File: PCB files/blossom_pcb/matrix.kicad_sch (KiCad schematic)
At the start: 136 parts, among them SW1 SW_Push, SW10 SW_Push, SW11 SW_Push, SW12 SW_Push, SW13 SW_Push, SW14 SW_Push, SW15 SW_Push, SW16 SW_Push, SW17 SW_Push, SW18 SW_Push, SW19 SW_Push, SW2 SW_Push, SW20 SW_Push, SW21 SW_Push, SW22 SW_Push, SW23 SW_Push, SW24 SW_Push, SW25 SW_Push, SW26 SW_Push, SW27 SW_Push, SW28 SW_Push, SW29 SW_Push, SW3 SW_Push, SW30 SW_Push, SW31 SW_Push, SW32 SW_Push, SW33 SW_Push, SW34 SW_Push, SW35 SW_Push, SW36 SW_Push, SW37 SW_Push, SW38 SW_Push, SW39 SW_Push, SW4 SW_Push, SW40 SW_Push, SW41 SW_Push, SW42 SW_Push, SW43 SW_Push, SW44 SW_Push, SW45 SW_Push, SW46 SW_Push, SW47 SW_Push, SW48 SW_Push, SW49 SW_Push, SW5 SW_Push, SW50 SW_Push, SW51 SW_Push, SW52 SW_Push, SW53 SW_Push, SW54 SW_Push, SW55 SW_Push, SW56 SW_Push, SW57 SW_Push, SW58 SW_Push, SW59 SW_Push, SW6 SW_Push, SW60 SW_Push, SW61 SW_Push, SW62 SW_Push, SW63 SW_Push, SW64 SW_Push, SW65 SW_Push, SW66 SW_Push, SW67 SW_Push, SW68 SW_Push, SW7 SW_Push, SW8 SW_Push, SW9 SW_Push

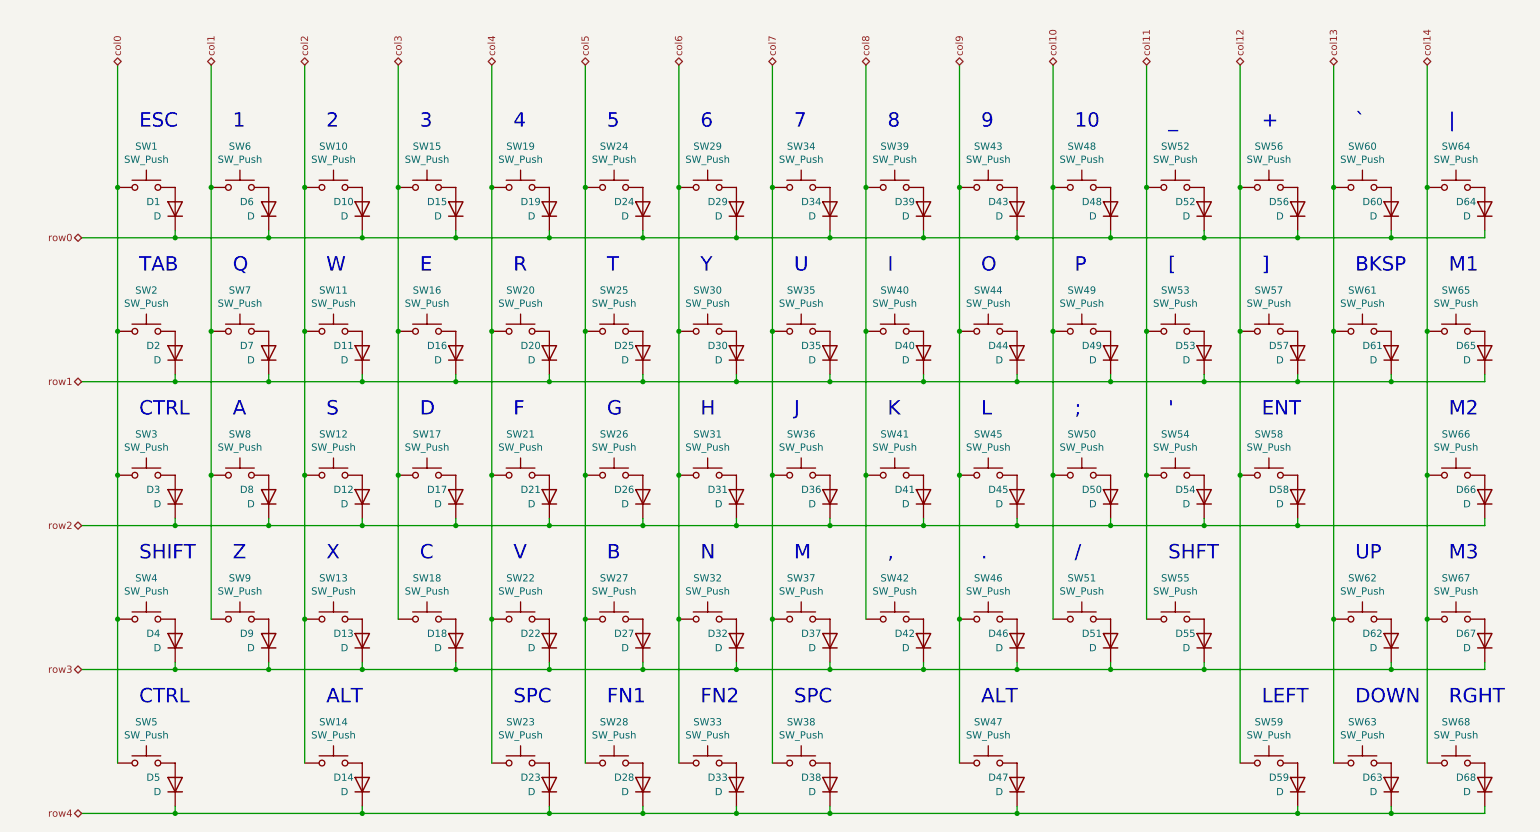
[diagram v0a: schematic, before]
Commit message: Almost doing stuffs
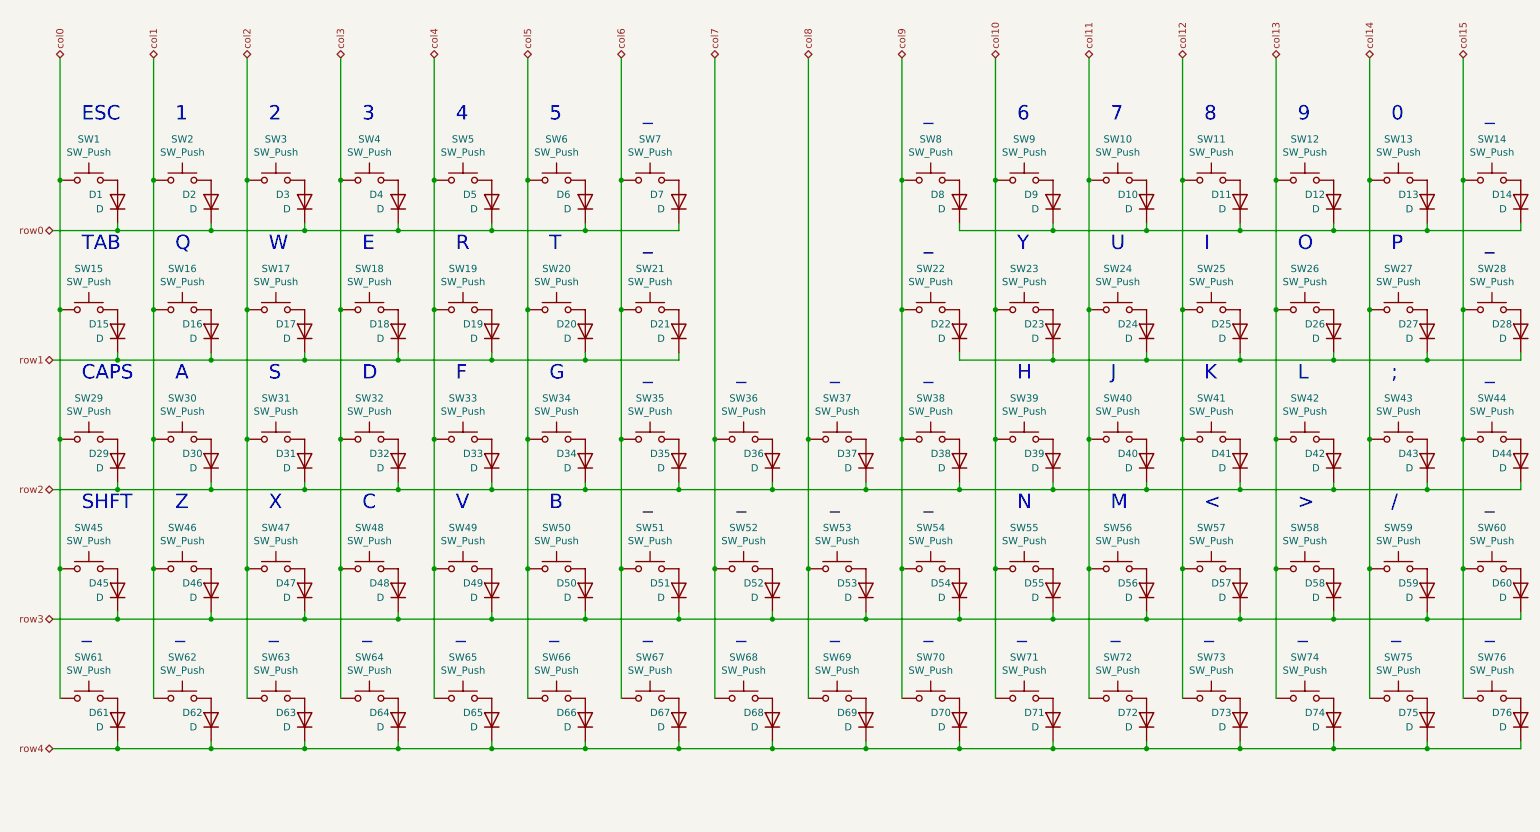
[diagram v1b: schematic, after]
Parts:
- removed D2, D3, D4, D5, D7: D, Diodes_SMD:D_SOD-123, symbol arisu-rescue:D-Device
- removed SW2, SW5: SW_Push, MX_Switch:SW_Cherry_MX_1.50u_PCB, symbol arisu-rescue:SW_Push-Switch
- removed SW3: SW_Push, MX_Switch:SW_Cherry_MX_1.75u_PCB, symbol arisu-rescue:SW_Push-Switch
- removed SW4: SW_Push, MX_Switch:SW_Cherry_MX_2.25u_PCB, symbol arisu-rescue:SW_Push-Switch
- removed SW7: SW_Push, MX_Switch:SW_Cherry_MX_1.00u_PCB, symbol arisu-rescue:SW_Push-Switch
- added D10, D15, D19, D24, D29, D69, D70, D71, D72, D73, D74, D75, D76: D, Diode_SMD:D_SOD-123, symbol arisu-rescue:D-Device
- added SW10, SW15, SW19, SW24, SW29, SW69, SW70, SW71, SW72, SW73, SW74, SW75, SW76: SW_Push, PCM_Switch_Keyboard_Hotswap_Kailh:SW_Hotswap_Kailh_MX_1.00u, symbol arisu-rescue:SW_Push-Switch
- D1, D11, D12, D13, D14, D16, D17, D18, D20, D21, D22, D23, D25, D26, D27, D28, D30, D31, D32, D33, D34, D35, D36, D37, D38, D39, D40, D41, D42, D43, D44, D45, D46, D47, D48, D49, D50, D51, D52, D53, D54, D55, D56, D57, D58, D59, D60, D61, D62, D63, D64, D65, D66, D67, D68, D8, D9: footprint Diodes_SMD:D_SOD-123 -> Diode_SMD:D_SOD-123
- D2: renamed from D6; footprint Diodes_SMD:D_SOD-123 -> Diode_SMD:D_SOD-123
- D3: renamed from D10; footprint Diodes_SMD:D_SOD-123 -> Diode_SMD:D_SOD-123
- D4: renamed from D15; footprint Diodes_SMD:D_SOD-123 -> Diode_SMD:D_SOD-123
- D5: renamed from D19; footprint Diodes_SMD:D_SOD-123 -> Diode_SMD:D_SOD-123
- D6: renamed from D24; footprint Diodes_SMD:D_SOD-123 -> Diode_SMD:D_SOD-123
- D7: renamed from D29; footprint Diodes_SMD:D_SOD-123 -> Diode_SMD:D_SOD-123
- SW1, SW11, SW12, SW13, SW16, SW17, SW18, SW20, SW21, SW22, SW25, SW26, SW27, SW28, SW30, SW31, SW32, SW33, SW34, SW35, SW36, SW37, SW39, SW40, SW41, SW42, SW43, SW44, SW45, SW46, SW48, SW49, SW50, SW51, SW52, SW53, SW54, SW56, SW57, SW59, SW60, SW62, SW63, SW64, SW65, SW66, SW67, SW68, SW8, SW9: footprint MX_Switch:SW_Cherry_MX_1.00u_PCB -> PCM_Switch_Keyboard_Hotswap_Kailh:SW_Hotswap_Kailh_MX_1.00u
- SW14, SW47, SW61: footprint MX_Switch:SW_Cherry_MX_1.50u_PCB -> PCM_Switch_Keyboard_Hotswap_Kailh:SW_Hotswap_Kailh_MX_1.00u
- SW2: renamed from SW6; footprint MX_Switch:SW_Cherry_MX_1.00u_PCB -> PCM_Switch_Keyboard_Hotswap_Kailh:SW_Hotswap_Kailh_MX_1.00u
- SW23: footprint MX_Switch:SW_Cherry_MX_2.00u_PCB_ReversedStabilizers -> PCM_Switch_Keyboard_Hotswap_Kailh:SW_Hotswap_Kailh_MX_1.00u
- SW3: renamed from SW10; footprint MX_Switch:SW_Cherry_MX_1.00u_PCB -> PCM_Switch_Keyboard_Hotswap_Kailh:SW_Hotswap_Kailh_MX_1.00u
- SW38: footprint MX_Switch:SW_Cherry_MX_2.75u_PCB_ReversedStabilizers -> PCM_Switch_Keyboard_Hotswap_Kailh:SW_Hotswap_Kailh_MX_1.00u
- SW4: renamed from SW15; footprint MX_Switch:SW_Cherry_MX_1.00u_PCB -> PCM_Switch_Keyboard_Hotswap_Kailh:SW_Hotswap_Kailh_MX_1.00u
- SW5: renamed from SW19; footprint MX_Switch:SW_Cherry_MX_1.00u_PCB -> PCM_Switch_Keyboard_Hotswap_Kailh:SW_Hotswap_Kailh_MX_1.00u
- SW55: footprint MX_Switch:SW_Cherry_MX_1.75u_PCB -> PCM_Switch_Keyboard_Hotswap_Kailh:SW_Hotswap_Kailh_MX_1.00u
- SW58: footprint MX_Switch:SW_Cherry_MX_2.25u_PCB_ReversedStabilizers -> PCM_Switch_Keyboard_Hotswap_Kailh:SW_Hotswap_Kailh_MX_1.00u
- SW6: renamed from SW24; footprint MX_Switch:SW_Cherry_MX_1.00u_PCB -> PCM_Switch_Keyboard_Hotswap_Kailh:SW_Hotswap_Kailh_MX_1.00u
- SW7: renamed from SW29; footprint MX_Switch:SW_Cherry_MX_1.00u_PCB -> PCM_Switch_Keyboard_Hotswap_Kailh:SW_Hotswap_Kailh_MX_1.00u
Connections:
- net col0: now also SW45.1, SW61.1, SW15.1, SW29.1
- net col1: now also SW16.1, SW30.1, SW46.1, SW62.1; no longer SW8.1, SW9.1
- net col10: now also SW23.1, SW39.1, SW55.1, SW9.1, SW71.1; no longer SW48.1, SW49.1, SW50.1, SW51.1
- net col11: now also SW40.1, SW56.1, SW10.1, SW24.1, SW72.1; no longer SW52.1, SW53.1, SW54.1, SW55.1
- net col12: now also SW11.1, SW25.1, SW41.1, SW73.1; no longer SW56.1, SW58.1, SW59.1
- net col13: now also SW12.1, SW26.1, SW42.1, SW58.1, SW74.1; no longer SW60.1, SW61.1, SW62.1, SW63.1
- net col14: now also SW13.1, SW27.1, SW43.1, SW59.1, SW75.1; no longer SW64.1, SW65.1, SW66.1, SW67.1, SW68.1
- net col2: now also SW17.1, SW31.1, SW47.1, SW63.1; no longer SW11.1, SW12.1, SW13.1, SW14.1
- net col3: now also SW32.1, SW48.1, SW64.1; no longer SW16.1, SW17.1
- net col4: now also SW33.1, SW49.1, SW65.1, SW19.1; no longer SW20.1, SW21.1, SW22.1, SW23.1
- net col5: now also SW20.1, SW34.1, SW50.1, SW66.1; no longer SW25.1, SW26.1, SW27.1, SW28.1
- net col6: now also SW21.1, SW35.1, SW51.1, SW67.1; no longer SW30.1, SW31.1, SW32.1, SW33.1
- net col7: now also SW52.1, SW68.1; no longer SW34.1, SW35.1, SW37.1, SW38.1
- net col8: now also SW37.1, SW53.1, SW69.1; no longer SW39.1, SW40.1, SW41.1, SW42.1
- net col9: now also SW22.1, SW38.1, SW54.1, SW8.1, SW70.1; no longer SW43.1, SW44.1, SW45.1, SW46.1, SW47.1
- net row0: no longer D34.1 (K), D39.1 (K), D43.1 (K), D48.1 (K), D52.1 (K), D56.1 (K), D60.1 (K), D64.1 (K)
- net row1: now also D17.1 (K), D18.1 (K), D21.1 (K), D15.1 (K), D19.1 (K); no longer D11.1 (K), D25.1 (K), D30.1 (K), D35.1 (K), D40.1 (K), D44.1 (K), D49.1 (K), D53.1 (K), D57.1 (K), D61.1 (K), D65.1 (K)
- net row2: now also D30.1 (K), D32.1 (K), D33.1 (K), D34.1 (K), D35.1 (K), D37.1 (K), D38.1 (K), D39.1 (K), D40.1 (K), D42.1 (K), D43.1 (K), D44.1 (K), D29.1 (K); no longer D12.1 (K), D17.1 (K), D21.1 (K), D26.1 (K), D45.1 (K), D50.1 (K), D54.1 (K), D58.1 (K), D66.1 (K), D8.1 (K)
- net row3: now also D45.1 (K), D47.1 (K), D48.1 (K), D49.1 (K), D50.1 (K), D52.1 (K), D53.1 (K), D54.1 (K), D56.1 (K), D57.1 (K), D58.1 (K), D59.1 (K), D60.1 (K); no longer D13.1 (K), D18.1 (K), D22.1 (K), D27.1 (K), D32.1 (K), D37.1 (K), D42.1 (K), D62.1 (K), D67.1 (K), D9.1 (K)
- net row4: now also D61.1 (K), D62.1 (K), D64.1 (K), D65.1 (K), D66.1 (K), D67.1 (K), D69.1 (K), D70.1 (K), D71.1 (K), D72.1 (K), D73.1 (K), D74.1 (K), D75.1 (K), D76.1 (K); no longer D14.1 (K), D23.1 (K), D28.1 (K), D33.1 (K), D38.1 (K), D47.1 (K), D59.1 (K)
- new net: D72.2 (A), SW72.2
- new net: D22.1 (K), D23.1 (K), D24.1 (K), D25.1 (K), D26.1 (K), D27.1 (K), D28.1 (K)
- new net: D29.2 (A), SW29.2
- new net: D73.2 (A), SW73.2
- new net: D70.2 (A), SW70.2
- new net: D10.1 (K), D11.1 (K), D12.1 (K), D13.1 (K), D14.1 (K), D8.1 (K), D9.1 (K)
- new net: D10.2 (A), SW10.2
- new net: D24.2 (A), SW24.2
- new net: D74.2 (A), SW74.2
- new net: D71.2 (A), SW71.2
- new net: D15.2 (A), SW15.2
- new net: D76.2 (A), SW76.2
- new net: D69.2 (A), SW69.2
- new net: D75.2 (A), SW75.2
- new net: D19.2 (A), SW19.2
- new net col15: SW14.1, SW28.1, SW44.1, SW60.1, SW76.1
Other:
- note added: "0"
- note added: "<"
- note added: ">"
- note added: "CAPS"
- note removed: "'"
- note removed: "+"
- note removed: ","
- note removed: "."
- note removed: "10"
- note removed: "ALT"
- note removed: "BKSP"
- note removed: "CTRL"
- note removed: "DOWN"
- note removed: "ENT"
- note removed: "FN1"
- note removed: "FN2"
- note removed: "LEFT"
- note removed: "M1"
- note removed: "M2"
- note removed: "M3"
- note removed: "RGHT"
- note removed: "SHIFT"
- note removed: "SPC"
- note removed: "UP"
- note removed: "["
- note removed: "]"
- note removed: "`"
- note removed: "|"
- moved on the sheet: D1, D2, D3, D4, D5, D6, D7, SW1, SW2, SW3, SW4, SW5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
